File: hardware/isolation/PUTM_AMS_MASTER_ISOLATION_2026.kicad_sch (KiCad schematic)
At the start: 7 parts, among them IC4 TLV61046ADBVT

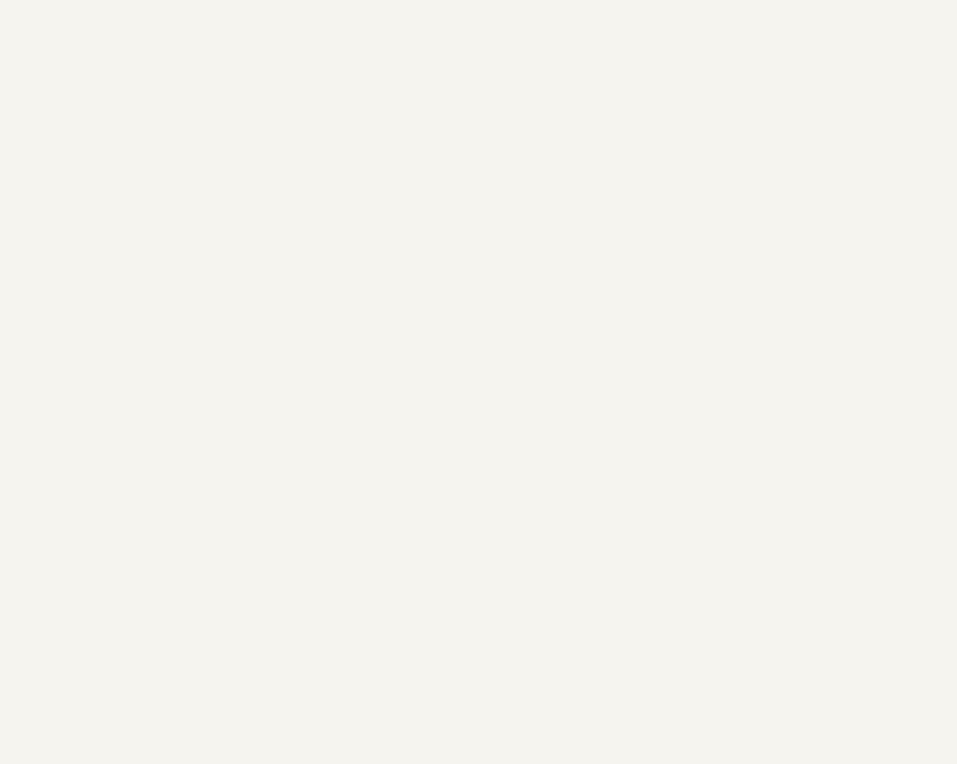
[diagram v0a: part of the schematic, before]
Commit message: chore: sync
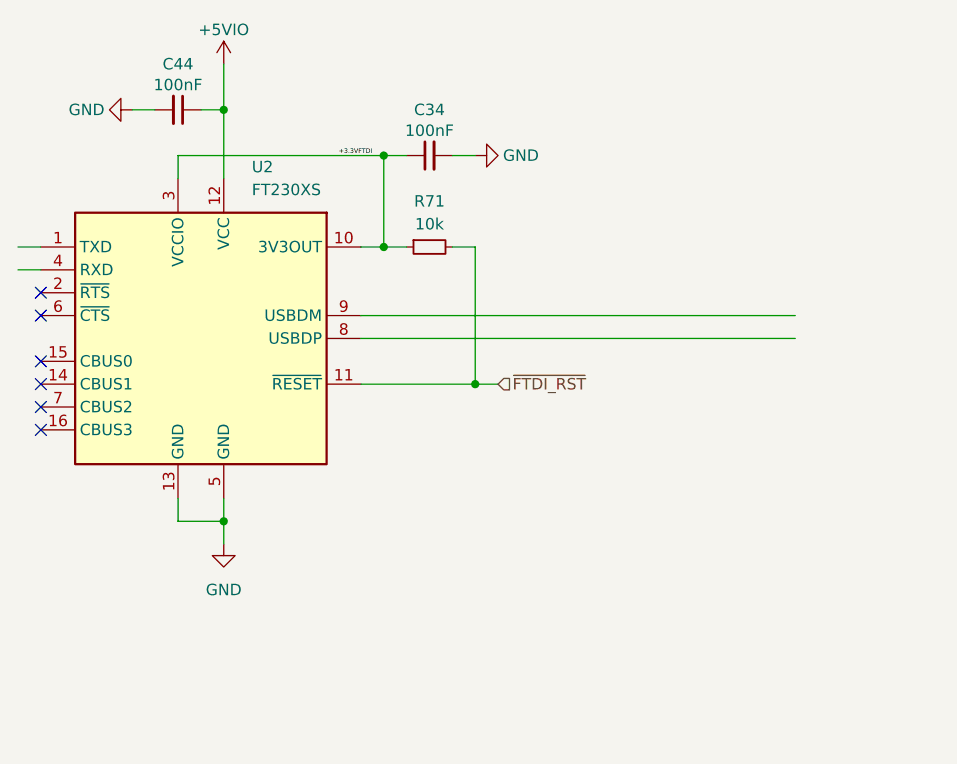
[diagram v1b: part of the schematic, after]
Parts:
- added C34, C44: 100nF, Capacitor_SMD:C_0603_1608Metric, symbol Device:C_Small
- added R71: 10k, Resistor_SMD:R_0603_1608Metric, symbol Device:R_Small
- added U2: FT230XS, Package_SO:SSOP-16_3.9x4.9mm_P0.635mm, symbol Interface_USB:FT230XS
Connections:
- net +5VIO: now also C44.1, U2.12 (VCC)
- net GND: now also C34.2, C44.2, U2.13 (GND), U2.5 (GND)
- new net +3.3VFTDI: C34.1, R71.1, U2.10 (3V3OUT), U2.3 (VCCIO)
- new net ~{FTDI_RST}: R71.2, U2.11 (~{RESET})
- no-connect marks 0 -> 6
